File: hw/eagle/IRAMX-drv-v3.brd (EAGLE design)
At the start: 55 x 75 mm, 59 parts, among them IC1 IRAMTOP, IC2 STM32F103R6T, IC3 78L05SMD, IC4 78L05SMD

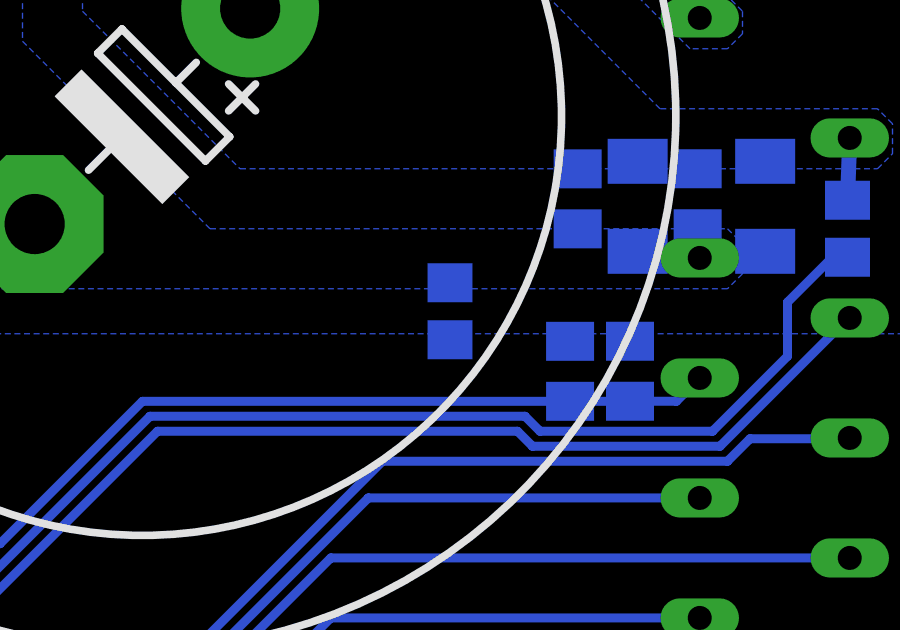
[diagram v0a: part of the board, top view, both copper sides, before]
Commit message: iramx v3
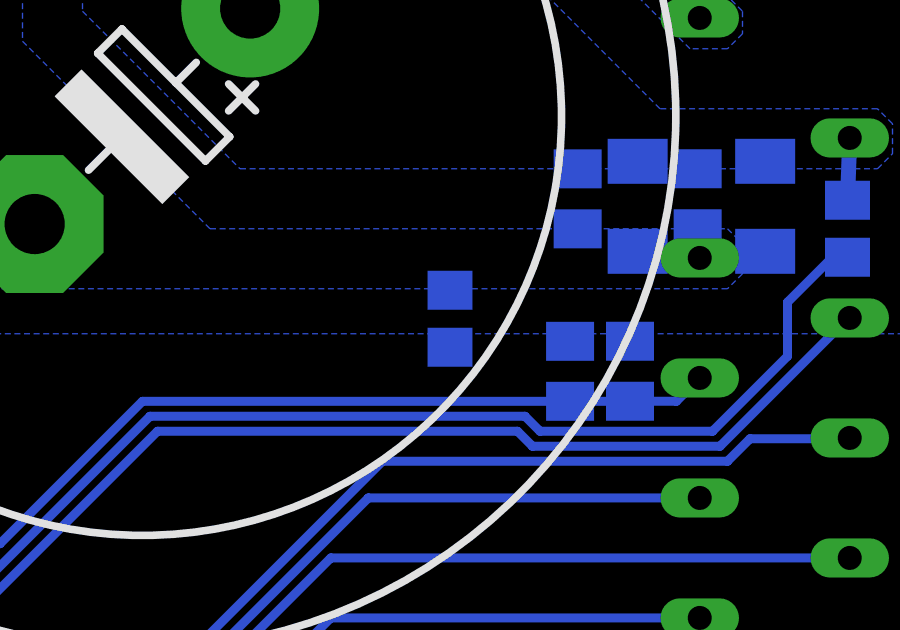
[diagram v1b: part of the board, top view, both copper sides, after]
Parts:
- moved R8 0.25 mm to (83.2, 41.0)
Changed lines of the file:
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@@
 <element name="C21" library="rcl" package="A/3216-18R" value="" x="57.25" y="58.75" rot="MR90"/>
 <element name="H4" library="holes" package="3,2-PAD" value="MOUNT-PAD-ROUND3.2" x="50" y="40"/>
-<element name="R8" library="rcl" package="R0805" value="" x="83.25" y="41.25" rot="MR90"/>
+<element name="R8" library="rcl" package="R0805" value="" x="83.25" y="41" rot="MR90"/>
 </elements>
 <signals>

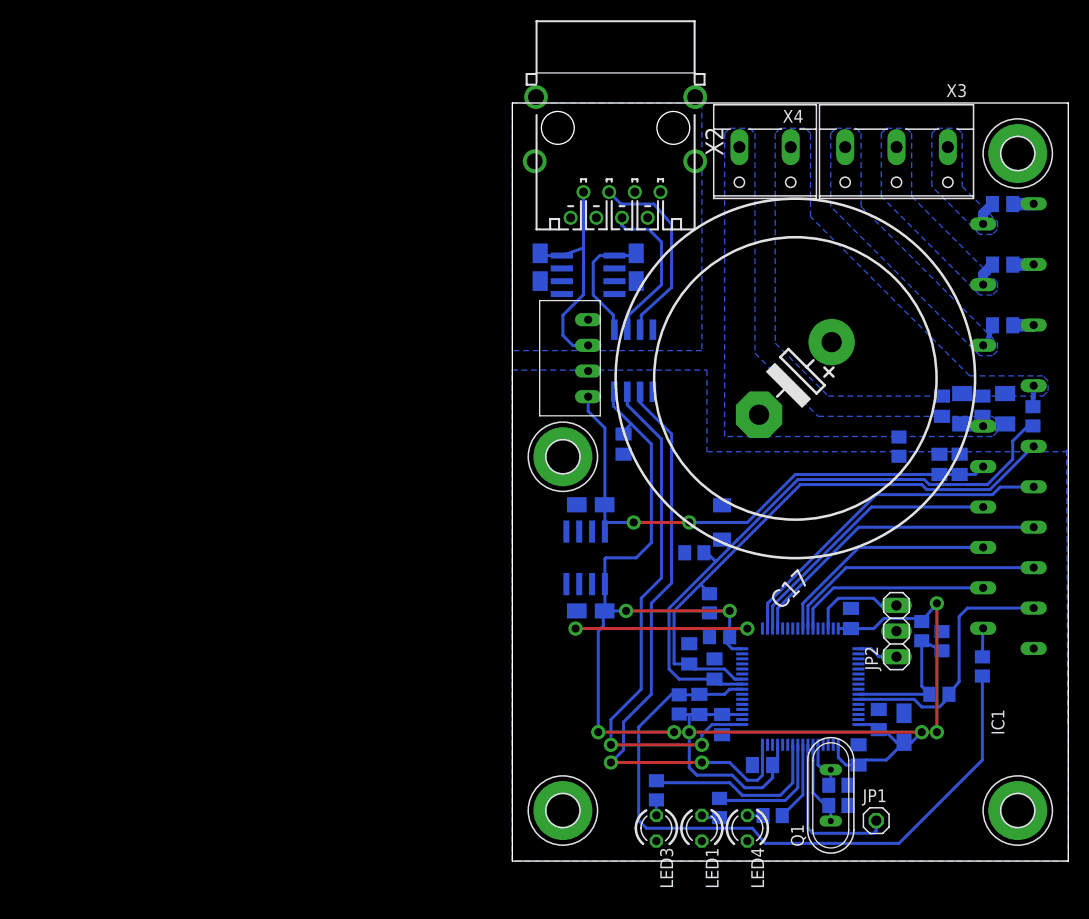
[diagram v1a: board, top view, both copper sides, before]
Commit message: iramx v3
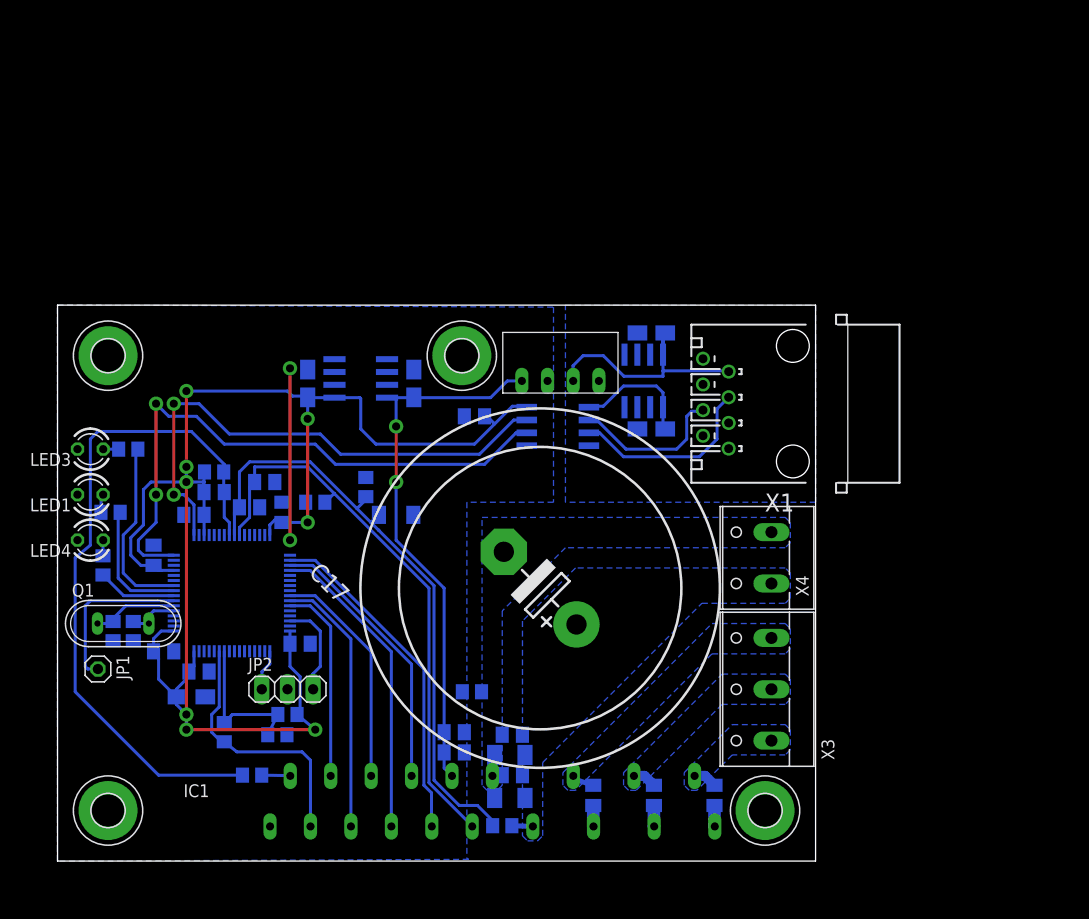
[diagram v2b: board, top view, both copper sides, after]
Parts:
- removed X2: (no value), con-appsys:RJ45
- added X1: (no value), reroolib:RJ45
- moved H2 90.0 mm to (5.00, 5.00), turned to 270 degrees
- moved JP1 78.4 mm to (4.00, 19.0), turned to 270 degrees
- moved C12 73.8 mm to (5.50, 22.8), turned to 90 degrees
- moved R11 73.0 mm to (19.3, 8.50), turned to 180 degrees
- moved Q1 72.0 mm to (6.50, 23.5), turned to 0 degrees
- moved C7 71.4 mm to (7.50, 22.8), turned to 90 degrees
- moved LED4 71.0 mm to (3.25, 31.8), turned to 180 degrees
- moved R23 70.8 mm to (16.5, 12.8), turned to 270 degrees
- moved R5 70.7 mm to (4.50, 29.2), turned to 270 degrees
- moved C28 70.6 mm to (13.2, 16.2), turned to 0 degrees
- moved H1 69.6 mm to (70.0, 5.00), turned to 270 degrees
- moved C18 69.5 mm to (10.5, 20.8), turned to 180 degrees
- moved LED1 68.9 mm to (3.25, 36.3), turned to 180 degrees
- moved C23 67.4 mm to (14.0, 18.8), turned to 180 degrees
- moved LED3 67.4 mm to (3.25, 40.8), turned to 180 degrees
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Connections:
- net ISO_GND: now also X1.8; no longer X2.8
- net N$13: now also X1.4; no longer X2.4
- net N$14: now also X1.5; no longer X2.5
- net N$17: now also X1.7; no longer X2.7
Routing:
- net N$17: track 22.6 -> 24.6 mm
- net N$14: track 19.6 -> 19.0 mm
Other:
- board size 55 x 75 mm -> 75 x 55 mm
